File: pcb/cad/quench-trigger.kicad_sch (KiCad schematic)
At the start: 34 parts, among them J701 Conn_Coaxial, J702 DB9_Female, K701 FINDER-30.22, Q701 BC846B, SW701 RST, SW702 TRIG, U701 74HCS08, U702 74HC574, U703 74LV132, U704 74LVC2G17, U705 74LVC2G17, U706 HFBR-1521Z

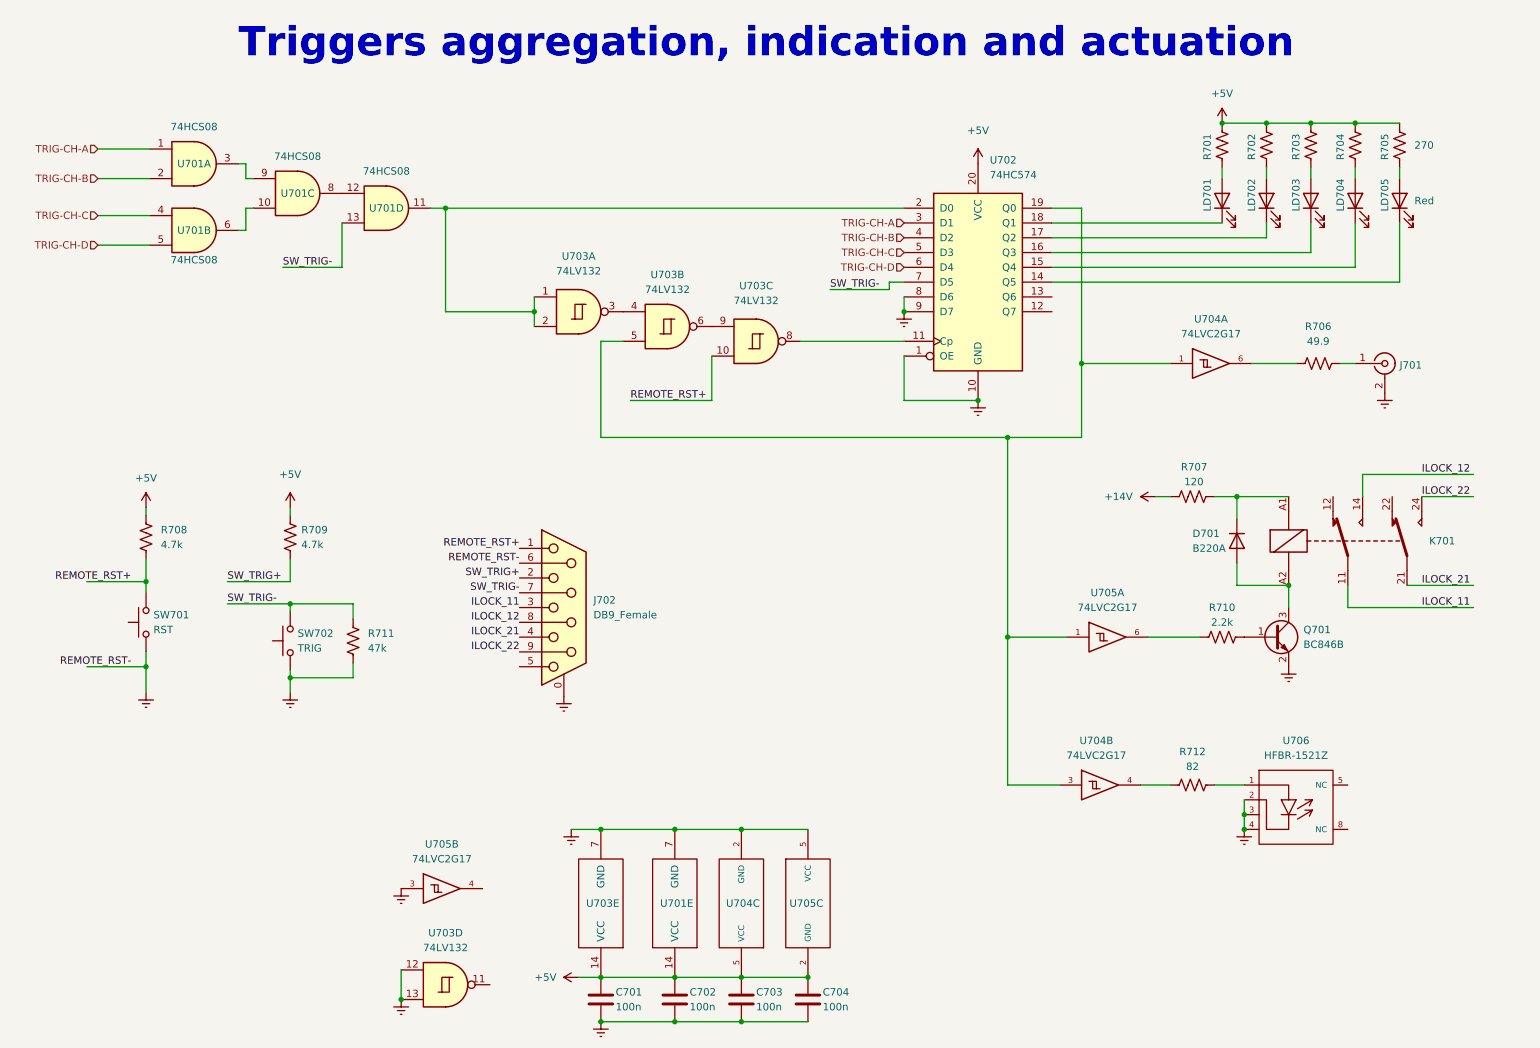
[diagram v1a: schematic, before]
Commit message: Place components of validation and quench trigger circuits on PCB
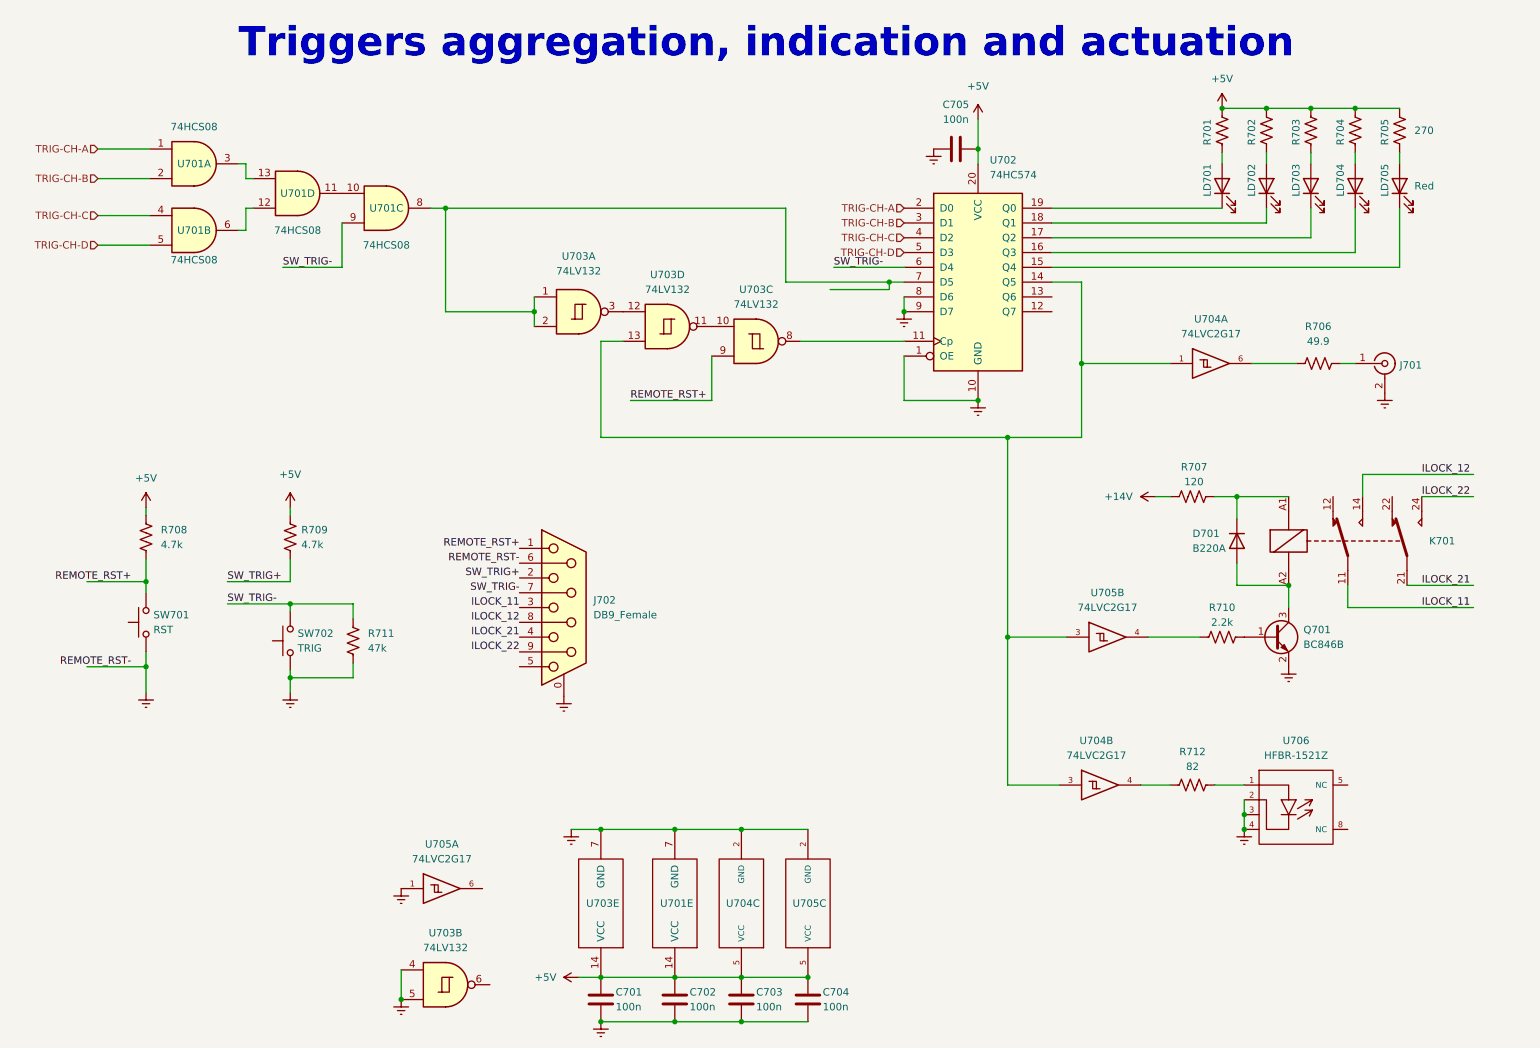
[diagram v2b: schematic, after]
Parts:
- added C705: 100n, Capacitor_SMD:C_0603_1608Metric_Pad1.08x0.95mm_HandSolder, symbol Device:C
- U702: footprint Package_SO:TSSOP-20_4.4x6.5mm_P0.65mm -> Package_SO:SO-20_12.8x7.5mm_P1.27mm
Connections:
- net +5V: now also U705.5 (VCC), C705.2; no longer U705.2 (GND)
- net Earth: now also U703.4, U703.5, U705.1, U705.2 (GND), C705.1; no longer U703.12, U703.13, U705.3, U705.5 (VCC)
- net REMOTE_RST+: now also U703.9; no longer U703.10
- net SW_TRIG-: now also U701.9, U702.6 (D4); no longer U701.13, U702.7 (D5)
- net TRIG-CH-A: now also U702.2 (D0); no longer U702.3 (D1)
- net TRIG-CH-B: now also U702.3 (D1); no longer U702.4 (D2)
- net TRIG-CH-C: now also U702.4 (D2); no longer U702.5 (D3)
- net TRIG-CH-D: now also U702.5 (D3); no longer U702.6 (D4)
- net at U705.4: now also R710.1
- net at U703.1, U703.2: now also U701.8, U702.7 (D5); no longer U701.11, U702.2 (D0)
- net at U703.3: now also U703.12; no longer U703.4
- net at U702.14 (Q5): now also U703.13, U704.1, U704.3, U705.3; no longer LD705.1 (K)
- net at U702.15 (Q4): now also LD705.1 (K); no longer LD704.1 (K)
- net at U702.16 (Q3): now also LD704.1 (K); no longer LD703.1 (K)
- net at U702.17 (Q2): now also LD703.1 (K); no longer LD702.1 (K)
- net at U702.18 (Q1): now also LD702.1 (K); no longer LD701.1 (K)
- net at U701.10: now also U701.11; no longer U701.6
- net at U701.12: now also U701.6; no longer U701.8
- net at U701.3: now also U701.13; no longer U701.9
- net at U703.11: now also U703.10
- net at U703.6: no longer U703.9
- net at U705.6: no longer R710.1
- new net: LD701.1 (K), U702.19 (Q0)
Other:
- moved on the sheet: LD701, LD702, LD703, LD704, LD705, R701, R702, R703, R704, R705, U701C, U701D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
